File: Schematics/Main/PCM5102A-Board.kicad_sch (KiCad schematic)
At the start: 7 parts, among them U3 PCM5102A, U4 MIC5219-3.3YM5, U5 MIC5219-3.3YM5

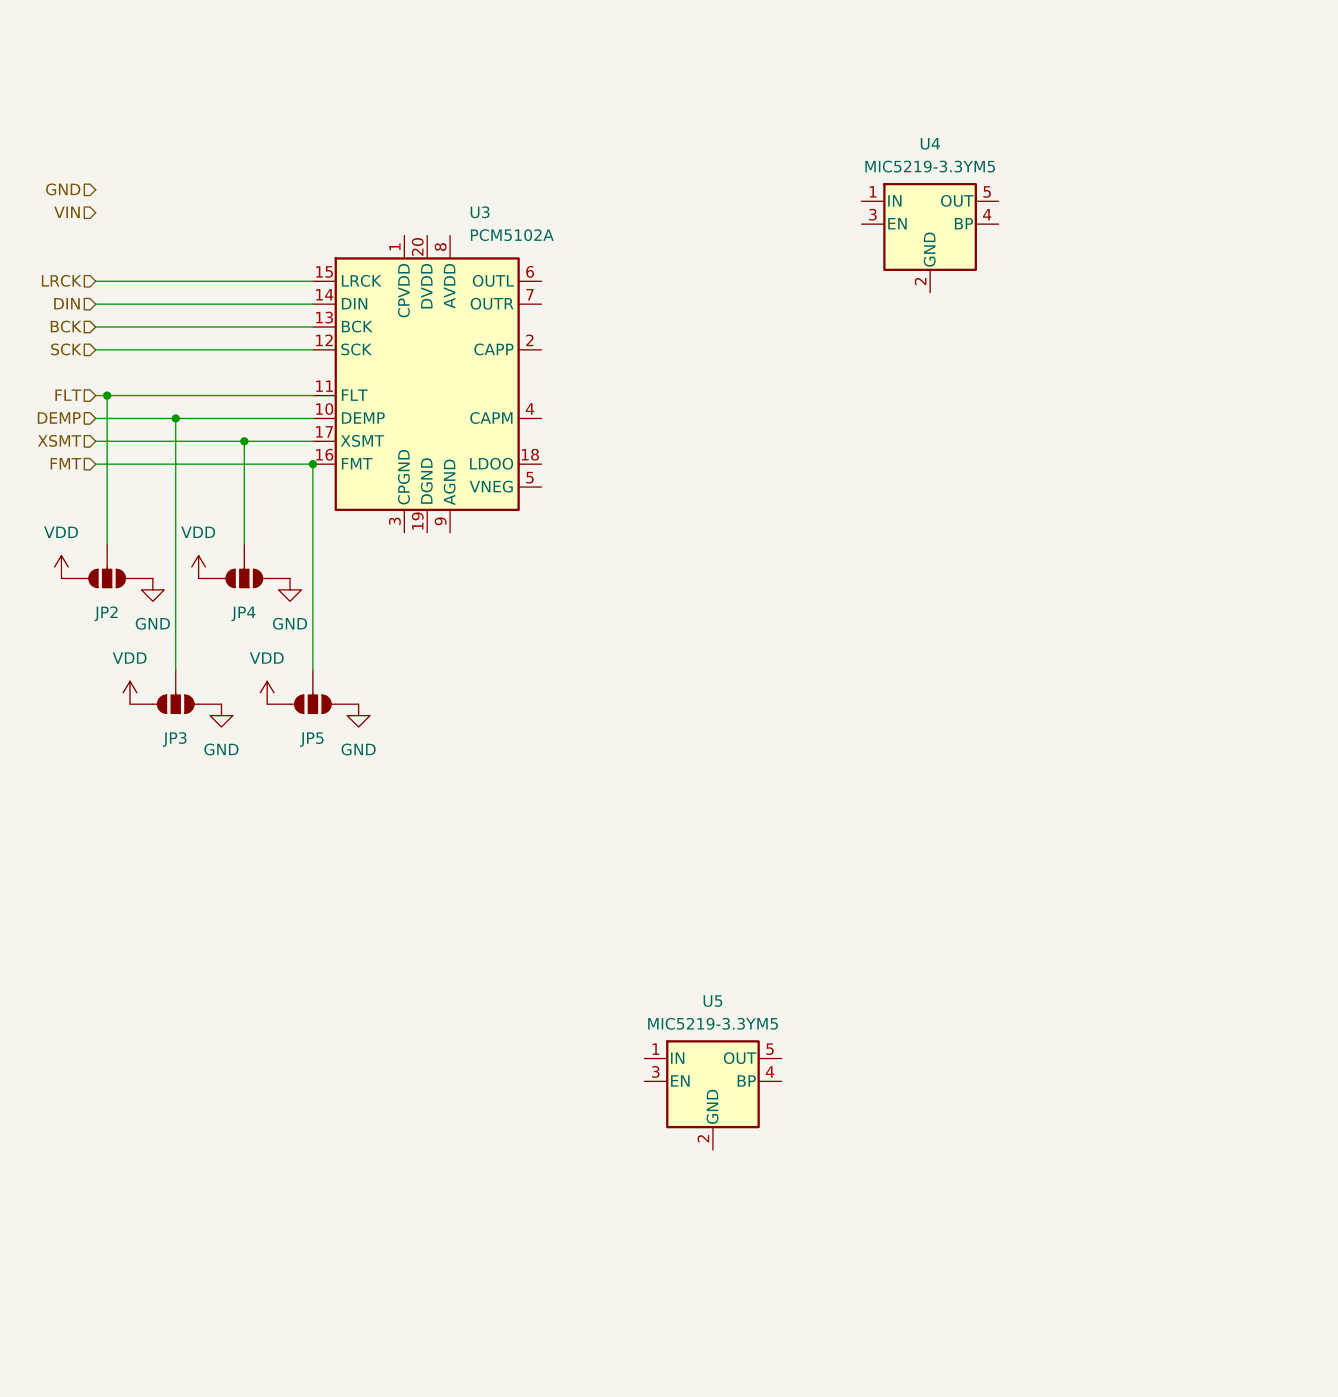
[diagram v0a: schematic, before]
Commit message: Added PCM5102A Board schematic
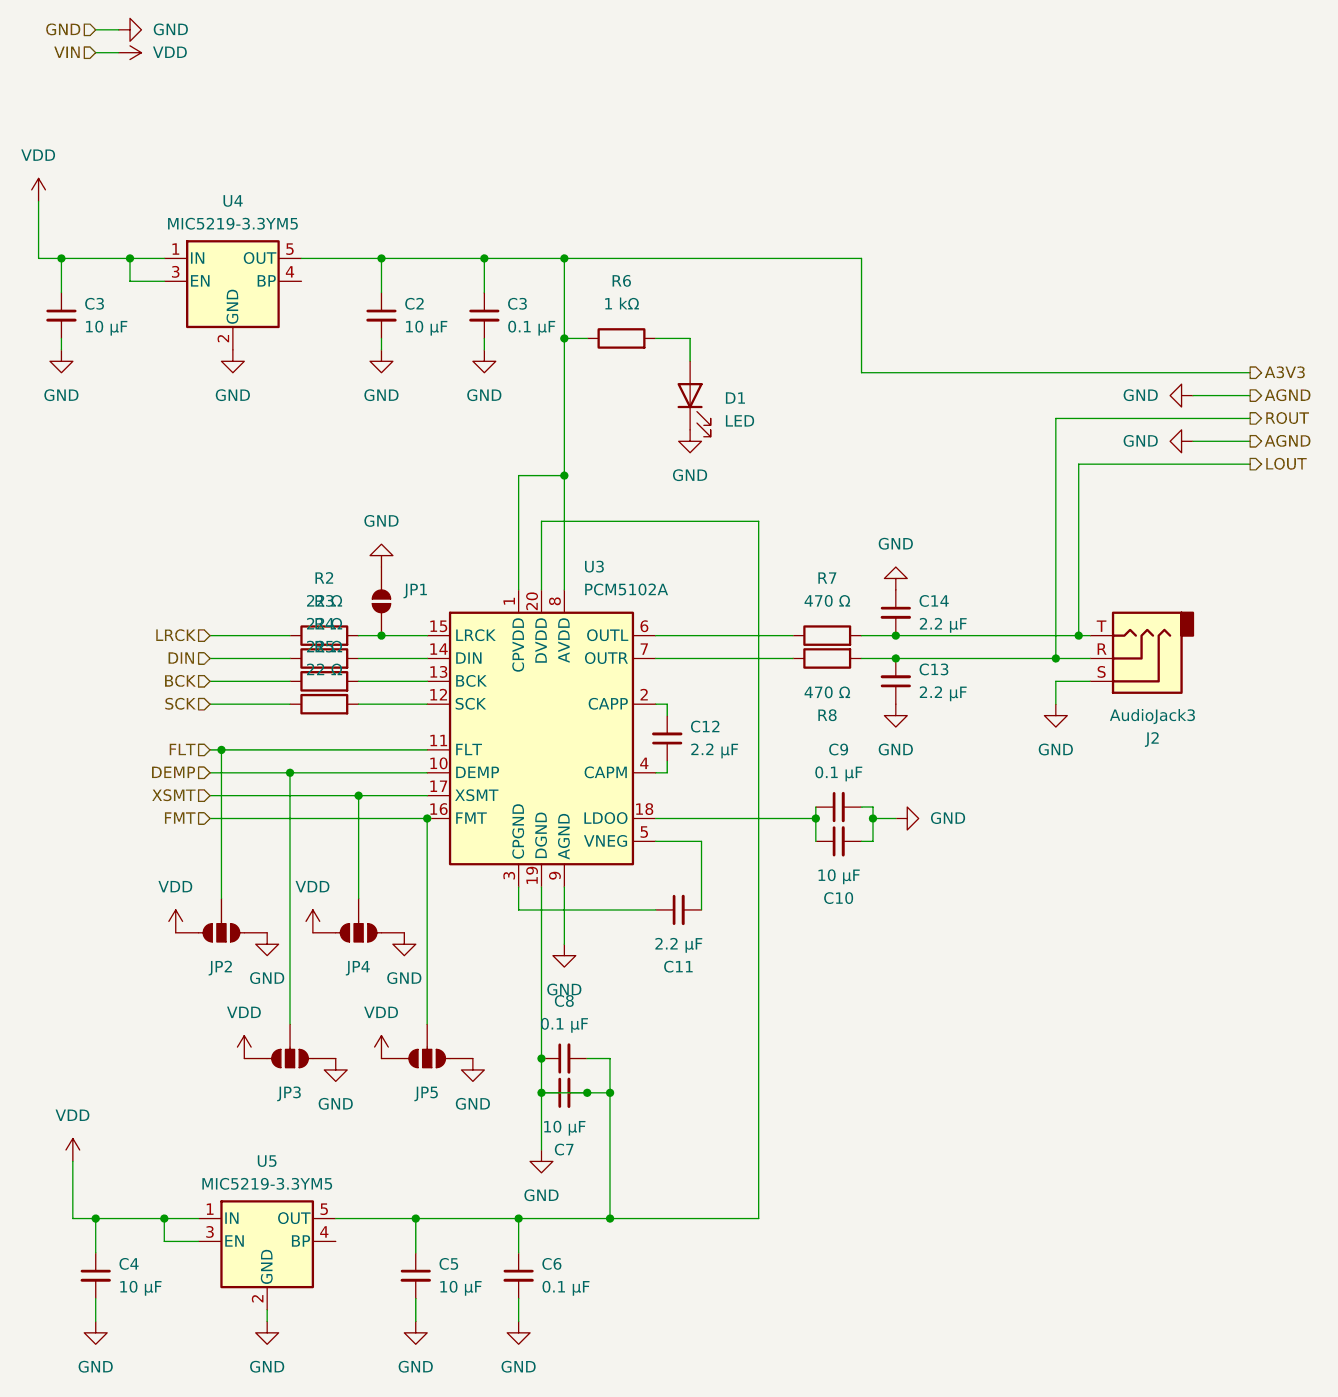
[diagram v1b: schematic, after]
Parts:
- added C10, C2, C3, C4, C5, C7: 10 μF, symbol Device:C_Small
- added C11, C12, C13, C14: 2.2 μF, symbol Device:C_Small
- added C3, C6, C8, C9: 0.1 μF, symbol Device:C_Small
- added D1: LED, symbol Device:LED
- added J2: AudioJack3, symbol Connector_Audio:AudioJack3
- added JP1: SolderJumper_2_Open, symbol Jumper:SolderJumper_2_Open
- added R2, R3, R4, R5: 22 Ω, symbol Device:R
- added R6: 1 kΩ, symbol Device:R
- added R7, R8: 470 Ω, symbol Device:R
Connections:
- net BCK: now also R4.1; no longer U3.13 (BCK)
- net DIN: now also R3.1; no longer U3.14 (DIN)
- net GND: now also U3.19 (DGND), U3.20 (DVDD), U3.9 (AGND), U4.2 (GND), U5.2 (GND), U5.5 (OUT), C10.2, C13.1, C14.1, C2.2, C3.2, C3.2, C4.2, C5.1, C5.2, C6.1, C6.2, C7.1, C7.2, C8.1, C8.2, C9.2, D1.1 (K), J2.S, JP1.2 (B)
- net LRCK: now also R2.1; no longer U3.15 (LRCK)
- net SCK: now also R5.1; no longer U3.12 (SCK)
- net VDD: now also U4.1 (IN), U4.3 (EN), U5.1 (IN), U5.3 (EN), C3.1, C4.1
- net A3V3: now reaches U3.1 (CPVDD)
- net A3V3: now also U3.8 (AVDD), U4.5 (OUT), C2.1, C3.1, R6.1
- net at U3.18 (LDOO): now also C10.1, C9.1
- net at U3.2 (CAPP): now also C12.2
- net at U3.3 (CPGND): now also C11.1
- net at U3.4 (CAPM): now also C12.1
- net at U3.5 (VNEG): now also C11.2
- net at U3.6 (OUTL): now also R7.1
- net at U3.7 (OUTR): now also R8.1
- new net: R4.2, U3.13 (BCK)
- new net: JP1.1 (A), R2.2, U3.15 (LRCK)
- new net: D1.2 (A), R6.2
- new net: R5.2, U3.12 (SCK)
- new net: R3.2, U3.14 (DIN)
- new net LOUT: C14.2, J2.T, R7.2
- new net ROUT: C13.2, J2.R, R8.2
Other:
- moved on the sheet: JP2, JP3, JP4, JP5, U3, U4
